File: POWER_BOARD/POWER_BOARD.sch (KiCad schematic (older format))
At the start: 38 parts, among them IC1 ILQ30, J1 EXTIN, J2 ARM, J3 Pyro1, J4 Pyro2, J5 Servo2, J6 Servo1, J7 Batt, J8 EXTIN, Q1 IRL40B212, Q2 IRL40B212, U1 SF-1206HH10M-2, U2 SF-1206HH10M-2, U3 AS358AP

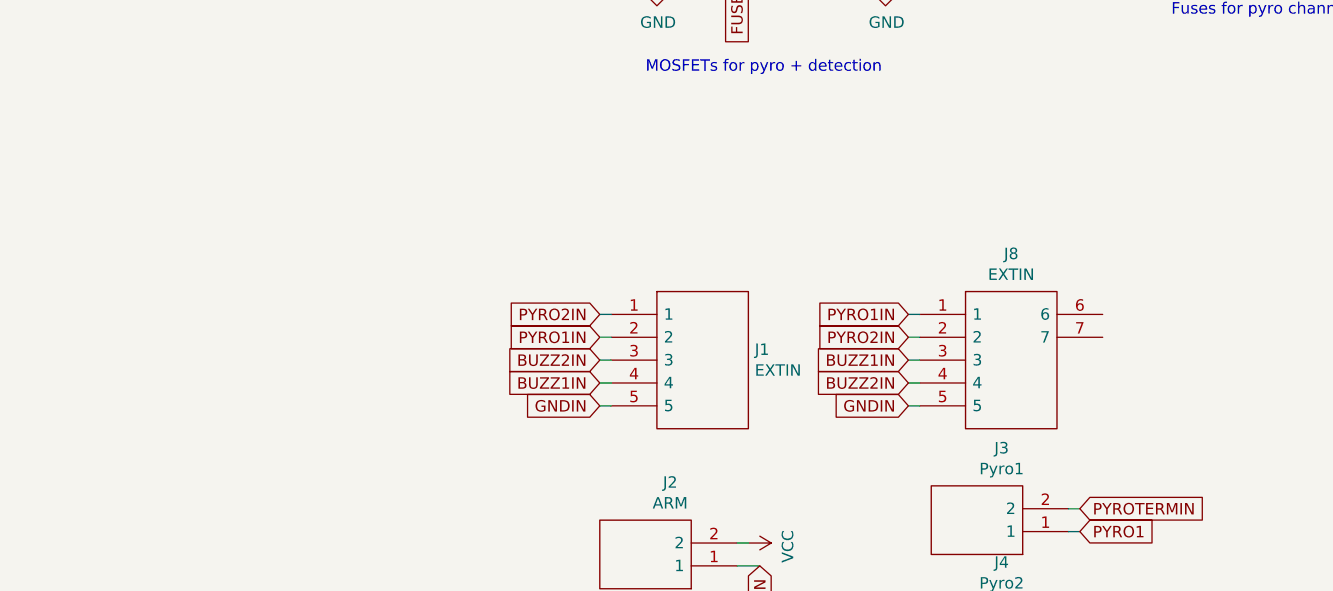
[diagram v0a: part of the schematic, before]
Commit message: t
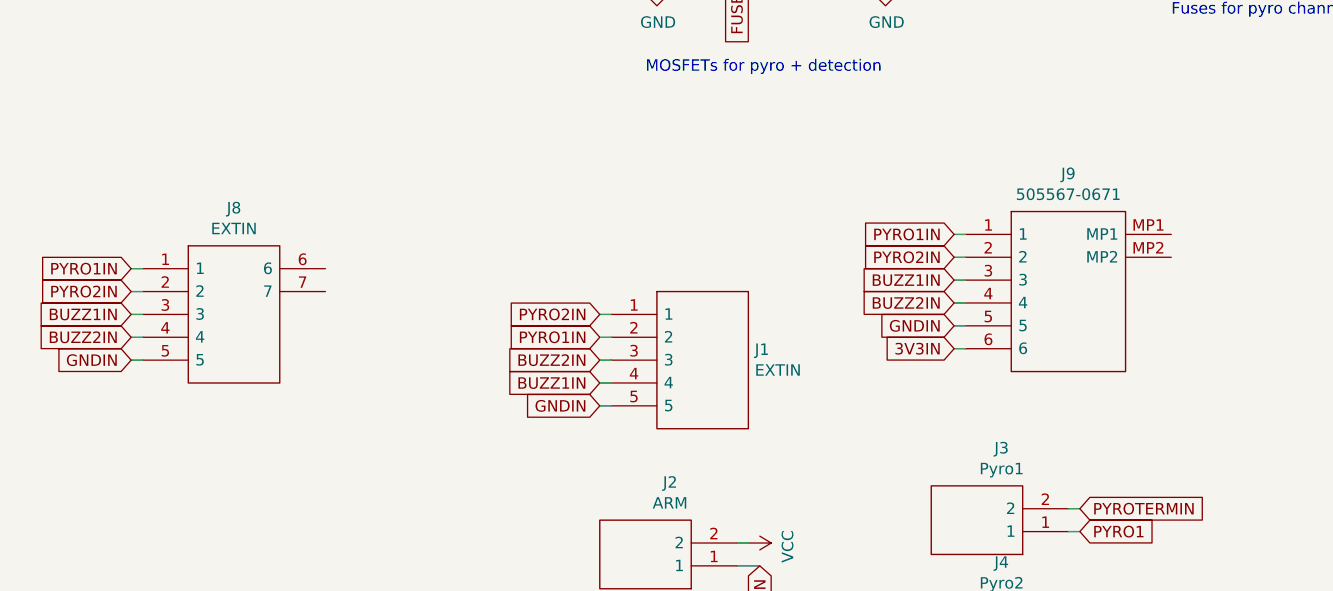
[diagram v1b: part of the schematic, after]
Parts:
- added J9: 505567-0671, EXTENSION:5055670671, symbol EXTENSION:505567-0671
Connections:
- net BUZZ1IN: now also J9.3
- net BUZZ2IN: now also J9.4
- net GNDIN: now also J9.5
- net PYRO1IN: now also J9.1
- net PYRO2IN: now also J9.2
- new net 3V3IN: J9.6
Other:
- moved on the sheet: J8
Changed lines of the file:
@@
 L EXTENSION:505567-0571 J8
 U 1 1 61909209
-P 2550 5100
-F 0 "J8" H 2950 5365 50  0000 C CNN
-F 1 "EXTIN" H 2950 5274 50  0000 C CNN
-F 2 "EXTENSION:5055670571" H 3200 5200 50  0001 L CNN
-F 3 "https://www.molex.com/pdm_docs/sd/5055670571_sd.pdf" H 3200 5100 50  0001 L CNN
-F 4 "Molex Micro-Lock PLUS 505567, 1.25mm Pitch, 5 Way, 1 Row, Right Angle PCB Header, Surface Mount" H 3200 5000 50  0001 L CNN "Description"
-F 5 "3" H 3200 4900 50  0001 L CNN "Height"
-F 6 "538-505567-0571" H 3200 4800 50  0001 L CNN "Mouser Part Number"
-F 7 "https://www.mouser.co.uk/ProductDetail/Molex/505567-0571?qs=gt1LBUVyoHnJxHrzoS78pw%3D%3D" H 3200 4700 50  0001 L CNN "Mouser Price/Stock"
-F 8 "Molex" H 3200 4600 50  0001 L CNN "Manufacturer_Name"
-F 9 "505567-0571" H 3200 4500 50  0001 L CNN "Manufacturer_Part_Number"
-	1    2550 5100
+P -850 4900
+F 0 "J8" H -450 5165 50  0000 C CNN
+F 1 "EXTIN" H -450 5074 50  0000 C CNN
+F 2 "EXTENSION:5055670571" H -200 5000 50  0001 L CNN
+F 3 "https://www.molex.com/pdm_docs/sd/5055670571_sd.pdf" H -200 4900 50  0001 L CNN
+F 4 "Molex Micro-Lock PLUS 505567, 1.25mm Pitch, 5 Way, 1 Row, Right Angle PCB Header, Surface Mount" H -200 4800 50  0001 L CNN "Description"
+F 5 "3" H -200 4700 50  0001 L CNN "Height"
+F 6 "538-505567-0571" H -200 4600 50  0001 L CNN "Mouser Part Number"
+F 7 "https://www.mouser.co.uk/ProductDetail/Molex/505567-0571?qs=gt1LBUVyoHnJxHrzoS78pw%3D%3D" H -200 4500 50  0001 L CNN "Mouser Price/Stock"
+F 8 "Molex" H -200 4400 50  0001 L CNN "Manufacturer_Name"
+F 9 "505567-0571" H -200 4300 50  0001 L CNN "Manufacturer_Part_Number"
+	1    -850 4900
 	1    0    0    -1
 $EndComp
-Text GLabel 2500 5100 0    50   Input ~ 0
+Text GLabel -900 4900 0    50   Input ~ 0
 PYRO1IN
-Text GLabel 2500 5200 0    50   Input ~ 0
+Text GLabel -900 5000 0    50   Input ~ 0
 PYRO2IN
-Text GLabel 2500 5300 0    50   Input ~ 0
+Text GLabel -900 5100 0    50   Input ~ 0
 BUZZ1IN
-Text GLabel 2500 5400 0    50   Input ~ 0
+Text GLabel -900 5200 0    50   Input ~ 0
 BUZZ2IN
-Text GLabel 2500 5500 0    50   Input ~ 0
+Text GLabel -900 5300 0    50   Input ~ 0
 GNDIN
 Wire Wire Line
-	2500 5500 2550 5500
+	-900 5300 -850 5300
 Wire Wire Line
-	2500 5400 2550 5400
+	-900 5200 -850 5200
 Wire Wire Line
-	2500 5300 2550 5300
+	-900 5100 -850 5100
 Wire Wire Line
-	2500 5200 2550 5200
+	-900 5000 -850 5000
 Wire Wire Line
-	2500 5100 2550 5100
+	-900 4900 -850 4900
 Text Notes 4850 2250 0    50   ~ 0
 LEDs debug
@@
 Text Notes 9050 2250 0    50   ~ 0
 Ampli OP for pyro detection
+Text GLabel 2700 4750 0    50   Input ~ 0
+PYRO1IN
+Text GLabel 2700 4850 0    50   Input ~ 0
+PYRO2IN
+Text GLabel 2700 4950 0    50   Input ~ 0
+BUZZ1IN
+Text GLabel 2700 5050 0    50   Input ~ 0
+BUZZ2IN
+Text GLabel 2700 5150 0    50   Input ~ 0
+GNDIN
+Wire Wire Line
+	2700 5150 2750 5150
+Wire Wire Line
+	2700 5050 2750 5050
+Wire Wire Line
+	2700 4950 2750 4950
+Wire Wire Line
+	2700 4850 2750 4850
+Wire Wire Line
+	2700 4750 2750 4750
+$Comp
+L EXTENSION:505567-0671 J9
+U 1 1 61BAC7D6
+P 2750 4750
+F 0 "J9" H 3200 5015 50  0000 C CNN
+F 1 "505567-0671" H 3200 4924 50  0000 C CNN
+F 2 "EXTENSION:5055670671" H 3500 4850 50  0001 L CNN
+F 3 "https://componentsearchengine.com/Datasheets/1/505567-0671.pdf" H 3500 4750 50  0001 L CNN
+F 4 "Molex Micro-Lock PLUS 505567, 1.25mm Pitch, 6 Way, 1 Row, Right Angle PCB Header, Surface Mount" H 3500 4650 50  0001 L CNN "Description"
+F 5 "4.2" H 3500 4550 50  0001 L CNN "Height"
+F 6 "538-505567-0671" H 3500 4450 50  0001 L CNN "Mouser Part Number"
+F 7 "https://www.mouser.co.uk/ProductDetail/Molex/505567-0671?qs=gt1LBUVyoHmQuimOt9l14w%3D%3D" H 3500 4350 50  0001 L CNN "Mouser Price/Stock"
+F 8 "Molex" H 3500 4250 50  0001 L CNN "Manufacturer_Name"
+F 9 "505567-0671" H 3500 4150 50  0001 L CNN "Manufacturer_Part_Number"
+	1    2750 4750
+	1    0    0    -1
+$EndComp
+Text GLabel 2700 5250 0    50   Input ~ 0
+3V3IN
+Wire Wire Line
+	2700 5250 2750 5250
 $EndSCHEMATC

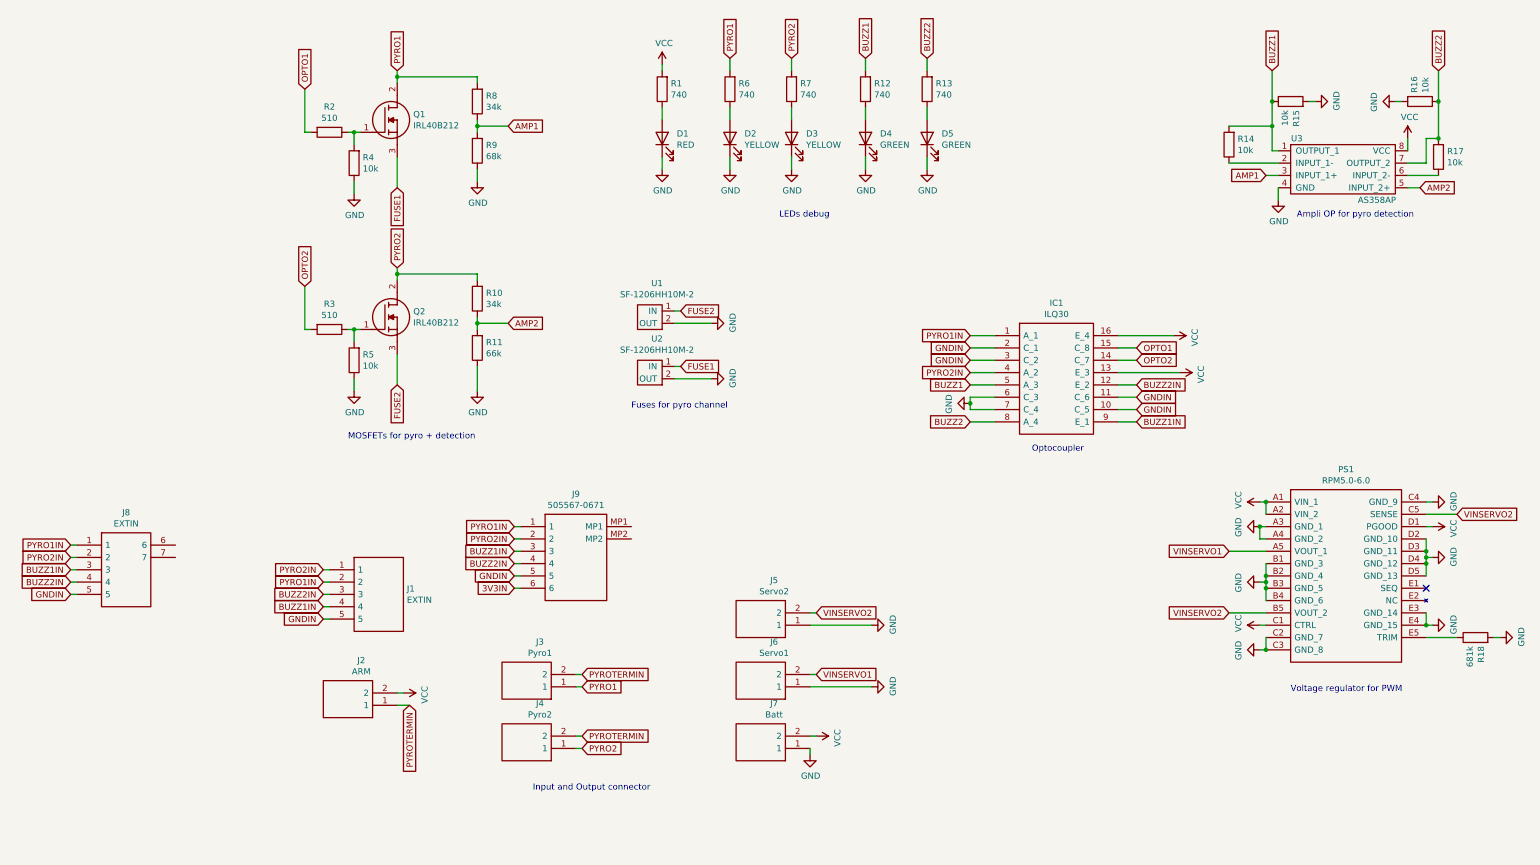
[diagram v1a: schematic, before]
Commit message: a
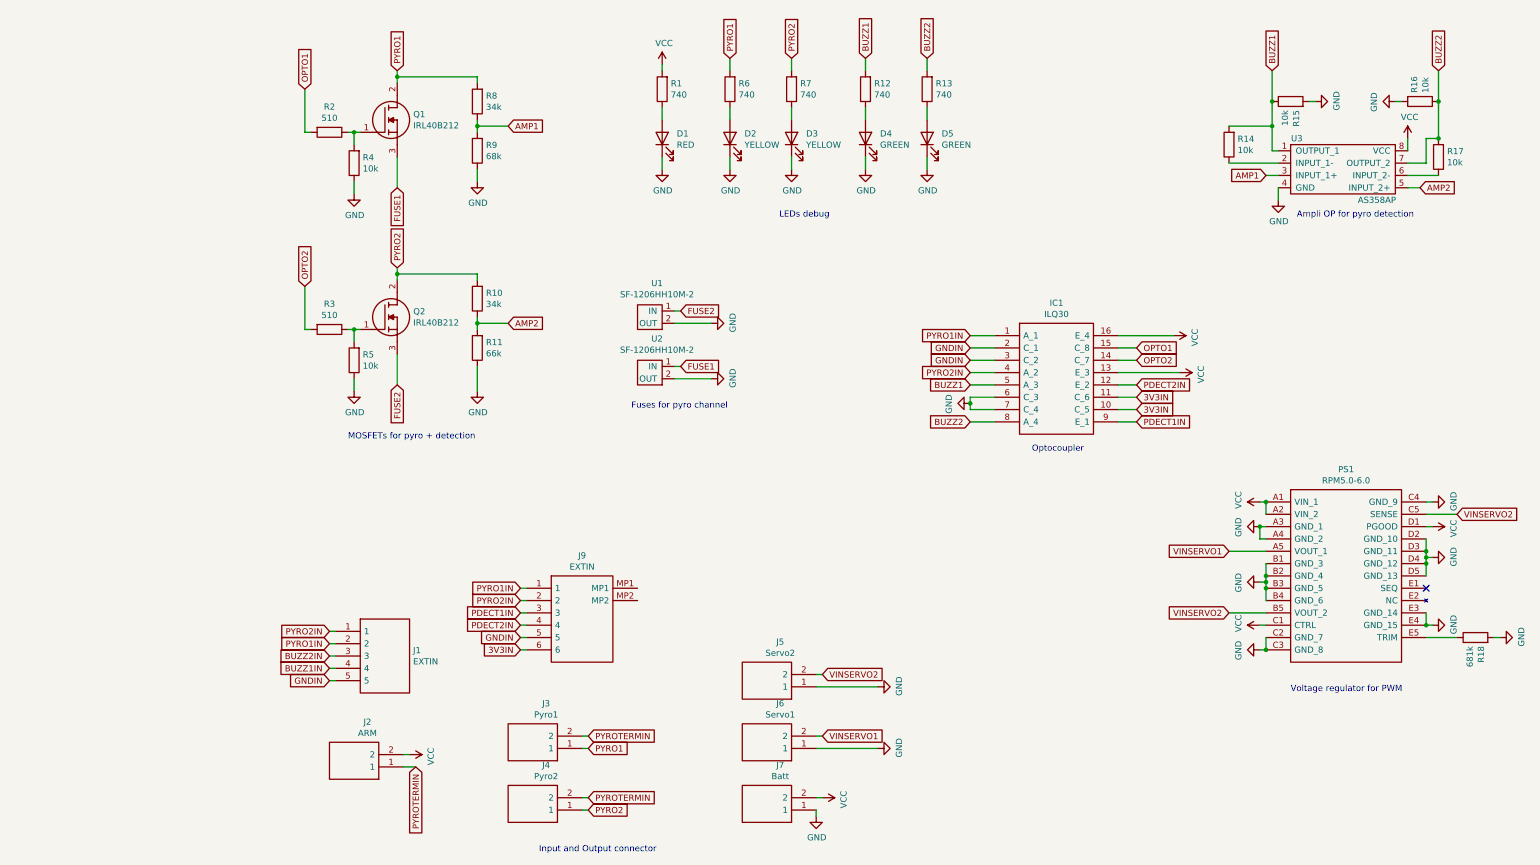
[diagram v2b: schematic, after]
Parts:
- removed J8: EXTIN, EXTENSION:5055670571, symbol EXTENSION:505567-0571
- J9: value 505567-0671 -> EXTIN
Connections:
- net 3V3IN: now also IC1.10 (C_5), IC1.11 (C_6)
- net BUZZ1IN: no longer IC1.9 (E_1), J9.3
- net BUZZ2IN: no longer IC1.12 (E_2), J9.4
- net GNDIN: no longer IC1.10 (C_5), IC1.11 (C_6)
- new net PDECT1IN: IC1.9 (E_1), J9.3
- new net PDECT2IN: IC1.12 (E_2), J9.4
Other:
- moved on the sheet: J1, J2, J3, J4, J5, J6, J7, J9
